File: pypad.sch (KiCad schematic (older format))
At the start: 59 parts, among them J1 Conn_01x05_Male, K1 SW_SPST, K10 SW_SPST, K11 SW_SPST, K12 SW_SPST, K13 SW_SPST, K14 SW_SPST, K15 SW_SPST, K16 SW_SPST, K17 SW_SPST, K18 SW_SPST, K19 SW_SPST, K2 SW_SPST, K20 SW_SPST, K3 SW_SPST, K4 SW_SPST, K5 SW_SPST, K6 SW_SPST, K7 SW_SPST, K8 SW_SPST, K9 SW_SPST, SW1 Rotary_Encoder_Switch, U1 BlackPill_F401RE

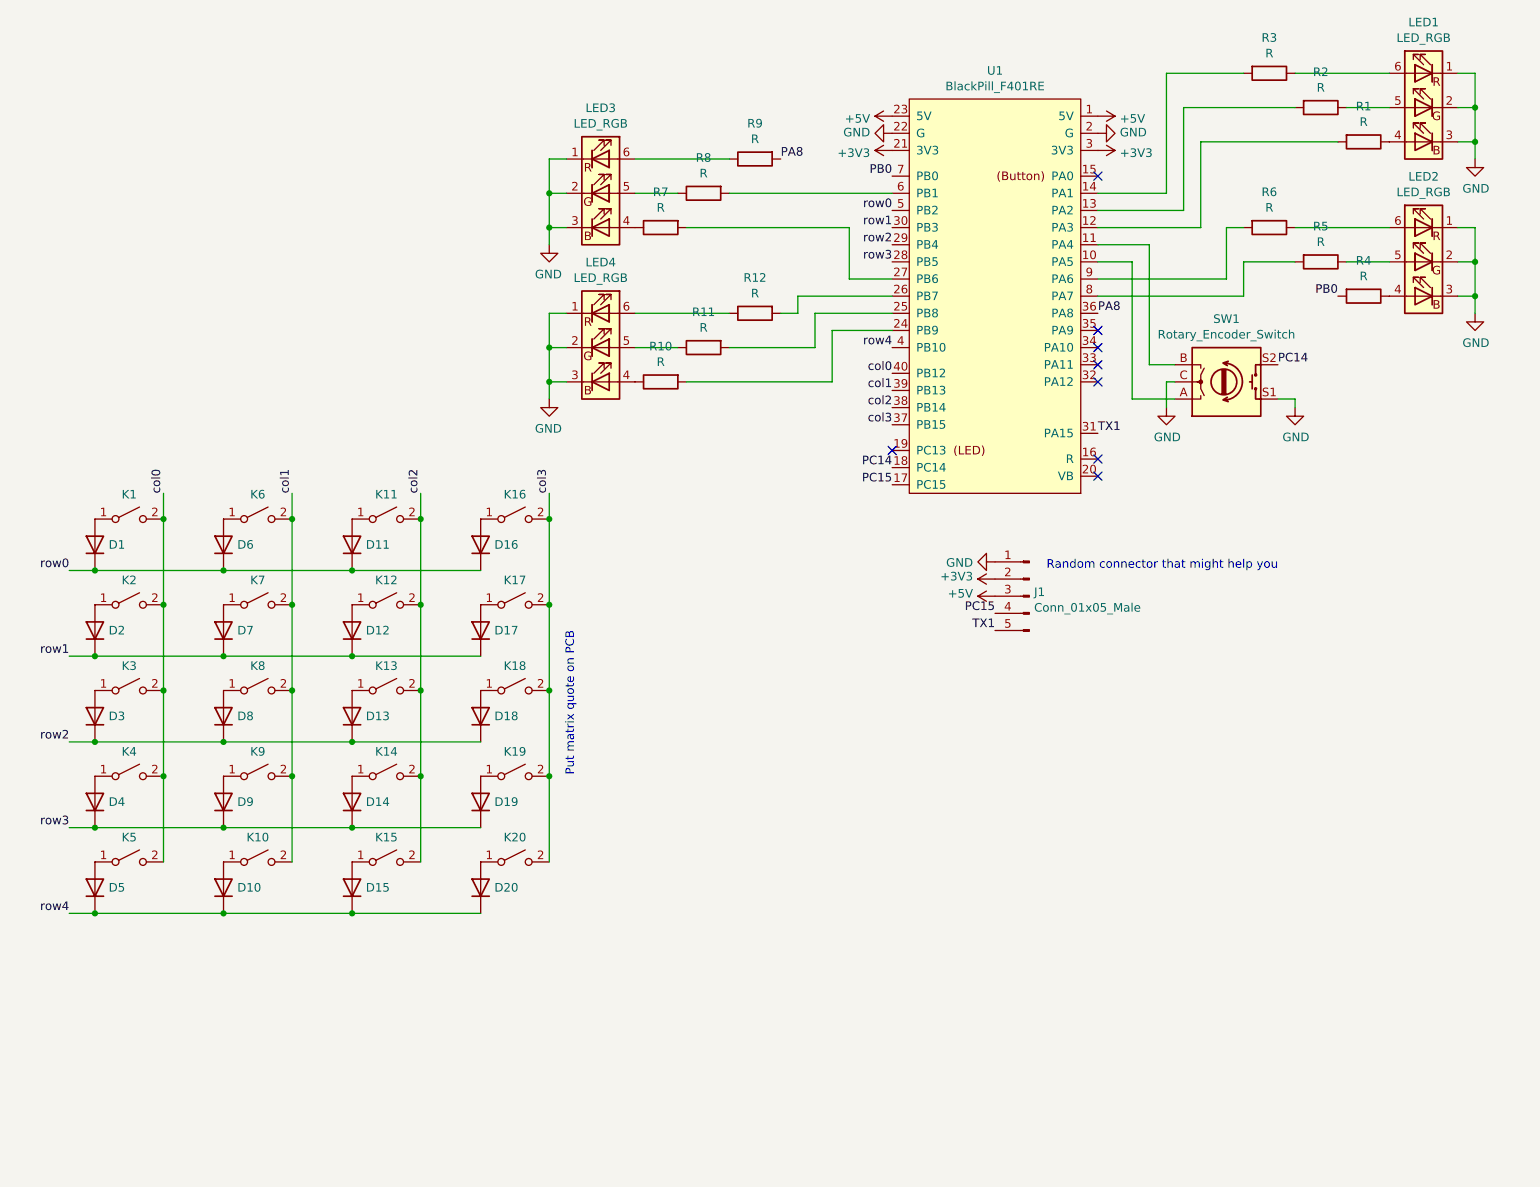
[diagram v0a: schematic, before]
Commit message: Routing attempt number 2
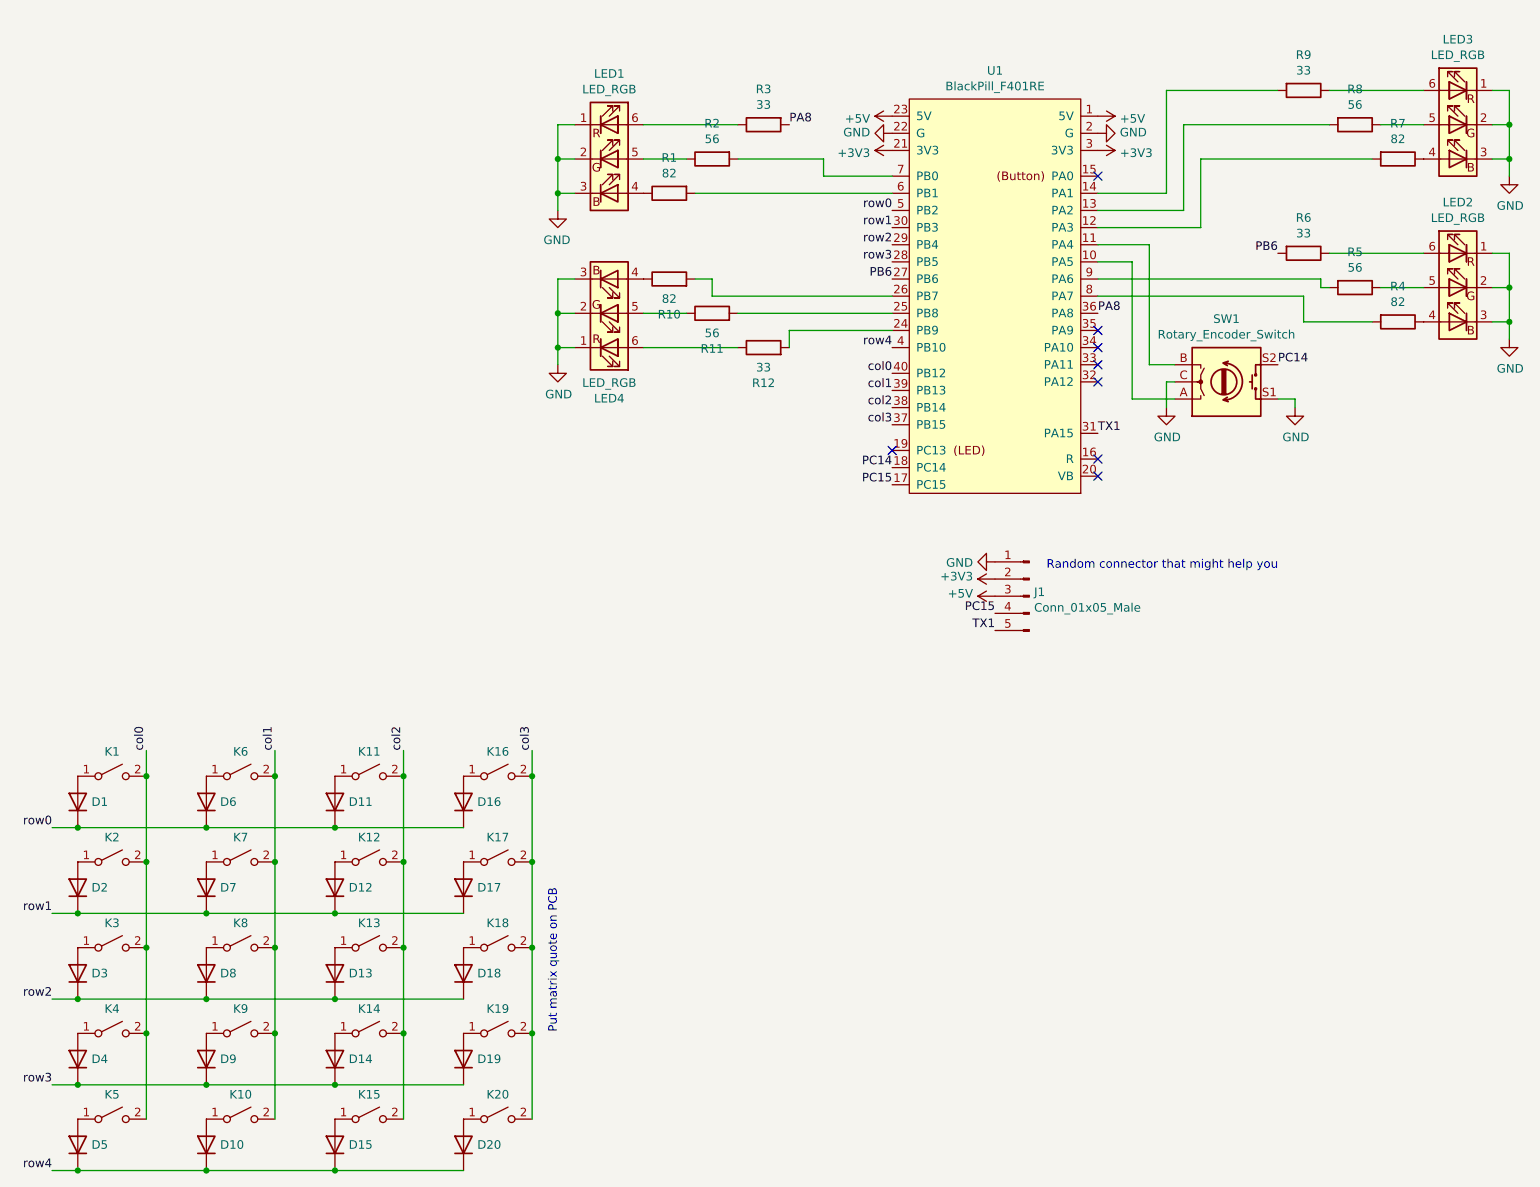
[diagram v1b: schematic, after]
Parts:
- D1, D10, D11, D12, D13, D14, D15, D16, D17, D18, D19, D2, D20, D3, D4, D5, D6, D7, D8, D9: footprint Diode_THT:D_DO-35_SOD27_P7.62mm_Horizontal -> PyPad_Footprints:D_DO-35_SOD27_P7.62mm_Horizontal
- K1, K10, K11, K12, K13, K14, K15, K16, K17, K18, K19, K2, K20, K3, K4, K5, K6, K7, K8, K9: footprint Button_Switch_Keyboard:SW_Cherry_MX_1.00u_PCB -> PyPad_Footprints:SW_Cherry_MX_1.00u_PCB
- R1, R10, R4, R7: value R -> 82
- R11, R2, R5, R8: value R -> 56
- R12, R3, R6, R9: value R -> 33
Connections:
- net PA8: now also R3.2; no longer R9.2
- net at U1.12 (PA3): now also R7.2; no longer R1.2
- net at U1.13 (PA2): now also R8.2; no longer R2.2
- net at U1.14 (PA1): now also R9.2; no longer R3.2
- net at U1.24 (PB9): now also R12.2; no longer R10.2
- net at U1.26 (PB7): now also R10.2; no longer R12.2
- net PB6: now reaches U1.27 (PB6)
- net PB6: now also R6.2; no longer R7.2
- net at U1.6 (PB1): now also R1.2; no longer R8.2
- net at U1.8 (PA7): now also R4.2; no longer R5.2
- net at U1.9 (PA6): now also R5.2; no longer R6.2
- net PB0: no longer names the net of U1.7 (PB0)
- net PB0: now also R2.2; no longer R4.2
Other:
- moved on the sheet: D1, D10, D11, D12, D13, D14, D15, D16, D17, D18, D19, D2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
